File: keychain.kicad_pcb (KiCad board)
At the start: 2 copper layers, 85.8 x 46 mm, 50 parts, among them Q1 PNP, Q10 NPN, Q11 NPN, Q12 NPN, Q13 PNP, Q14 PNP, Q15 NPN, Q16 NPN, Q17 PNP, Q18 PNP, Q19 NPN, Q2 PNP, Q20 NPN, Q21 NPN, Q22 NPN, Q3 PNP, Q4 PNP, Q5 PNP, Q6 PNP, Q7 PNP, Q8 NPN, Q9 NPN, SW1 SW_Push, SW2 SW_Push

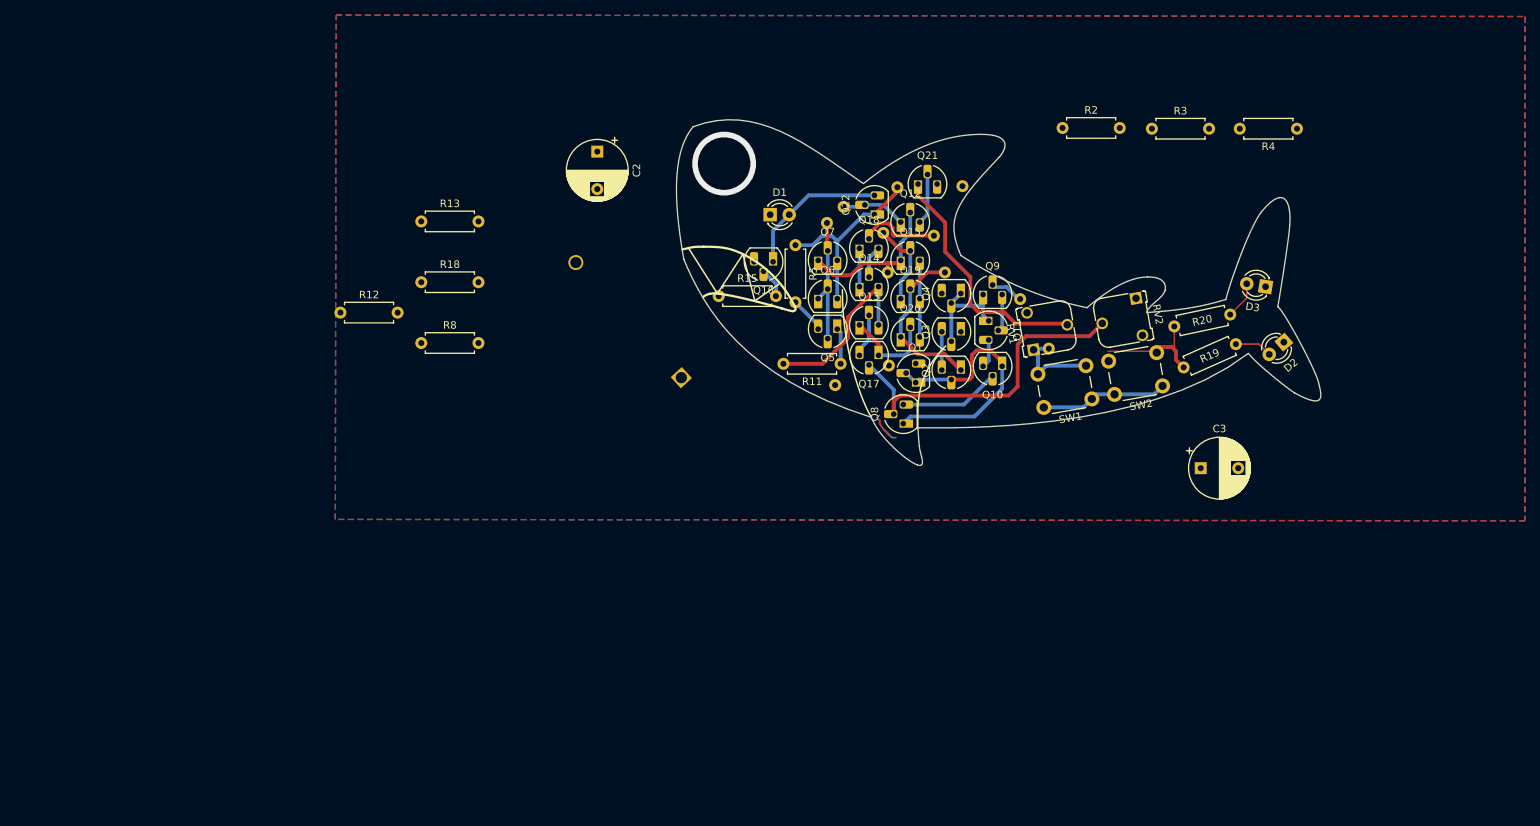
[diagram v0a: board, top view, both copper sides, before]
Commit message: Sync
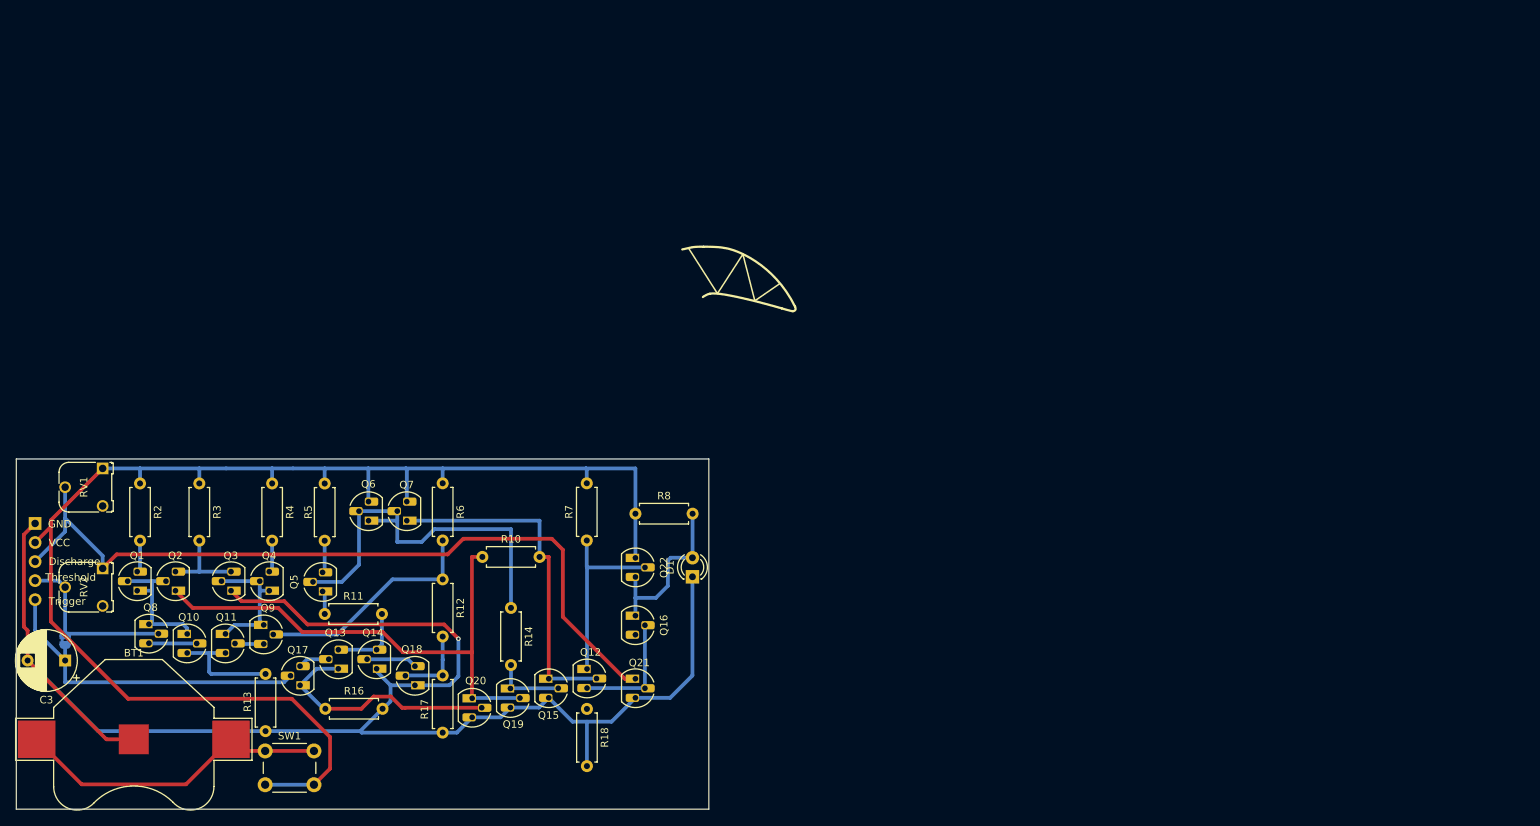
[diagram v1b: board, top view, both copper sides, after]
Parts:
- removed C2: C, Capacitor_THT:CP_Radial_D8.0mm_P5.00mm
- removed D2, D3: LED, LED_THT:LED_D3.0mm
- removed R15: 0ohm, Resistor_THT:R_Axial_DIN0207_L6.3mm_D2.5mm_P7.62mm_Horizontal
- removed R19, R20: R, Resistor_THT:R_Axial_DIN0207_L6.3mm_D2.5mm_P7.62mm_Horizontal
- removed SW2: SW_Push, Button_Switch_THT:SW_PUSH_6mm
- added J1: Conn_01x05_Pin, Connector_PinHeader_2.54mm:PinHeader_1x05_P2.54mm_Vertical, B.Cu at (21.6, 130.8)
- added JP1: SolderJumper_2_Bridged, Jumper:SolderJumper-2_P1.3mm_Bridged2Bar_RoundedPad1.0x1.5mm, B.Cu at (25.6, 146.4)
- BT1: footprint Battery:BatteryHolder_MYOUNG_BS-07-A1BJ001_CR2032 -> Battery:BatteryHolder_Multicomp_BC-2001_1x2032; moved to F.Cu
- R10, R14, R16, R17, R6, R7: moved to F.Cu
- moved C3 153.4 mm to (25.6, 149.1), turned to 180 degrees
- moved R4 144.5 mm to (53.2, 125.5), turned to -90 degrees
- moved RV2 142.3 mm to (30.6, 136.8), turned to -90 degrees
- moved R3 135.4 mm to (43.5, 125.5), turned to -90 degrees
- moved R2 131.7 mm to (35.6, 125.5), turned to -90 degrees
- moved RV1 125.0 mm to (30.6, 123.5), turned to -90 degrees
- moved SW1 119.7 mm to (52.3, 161.2), turned to 0 degrees
- moved Q10 114.3 mm to (41.9, 145.6), turned to -90 degrees
- moved Q11 109.9 mm to (47.0, 145.6)
- moved Q2 108.7 mm to (40.3, 139.8), turned to 90 degrees
- moved Q1 107.4 mm to (35.2, 139.8)
- moved Q9 105.5 mm to (52.1, 144.4), turned to -90 degrees
- moved Q8 104.0 mm to (36.8, 144.3), turned to -90 degrees
- moved Q3 103.2 mm to (47.7, 139.8), turned to 90 degrees
- moved Q4 100.3 mm to (52.8, 139.8), turned to 90 degrees
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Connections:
- C3 pad 1: THRESHOLD -> TRIGGER
- Q16 pad 2: Net-(Q16-B) -> Net-(Q12-E)
- Q17 pad 2: THRESHOLD -> TRIGGER
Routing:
- net GND: track 22.4 -> 213.3 mm, vias 0 -> 1
- net Net-(J1-Pin_2): track 38.3 -> 188.2 mm
- net DISCHARGE: track 32.8 -> 105.9 mm
- net Net-(Q19-B): track 22.3 -> 69.5 mm
- net TRIGGER: track 0.00 -> 45.1 mm
- net Net-(Q5-B): track 17.3 -> 53.7 mm
- net Net-(Q9-B): track 4.45 -> 30.8 mm
- net Net-(Q12-B): track 20.8 -> 46.4 mm
- net VCC: track 17.0 -> 42.6 mm
- net THRESHOLD: track 45.0 -> 23.0 mm
- net Net-(Q13-C): track 12.7 -> 32.8 mm
- net Net-(Q1-B): track 36.1 -> 19.4 mm
- net Net-(Q12-C): track 8.66 -> 24.9 mm
- net Net-(R19-Pad1): track 14.5 -> 0.00 mm
- net Net-(Q13-E): track 23.7 -> 10.2 mm
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- removed copper zone on B.Cu, net GND
- removed copper zone on F.Cu, net GND
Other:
- board size 85.8 x 46 mm -> 92.3 x 46.7 mm
- board text added: "1/3"
- board text added: "2/3"
- board text added: "Discharge"
- board text added: "GND"
- board text added: "Open 555"
- board text added: "Output"
- board text added: "SR Latch"
- board text added: "Threshold"
- board text added: "Threshold OPAmp"
- board text added: "Trigger"
- board text added: "Trigger OPAmp"
- board text added: "VCC"
- board text added: "Voltage devider"
